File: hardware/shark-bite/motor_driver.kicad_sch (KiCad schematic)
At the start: 53 parts, among them J2 Conn_ARM_SWD_TagConnect_TC203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, J3 PWM Pads, J6 Motor Pads, U10 SISS54, U11 SISS54, U12 SISS54, U2 DRV8300DRGER, U4 GD32E230G6U6TR, U7 SISS54, U8 SISS54, U9 SISS54

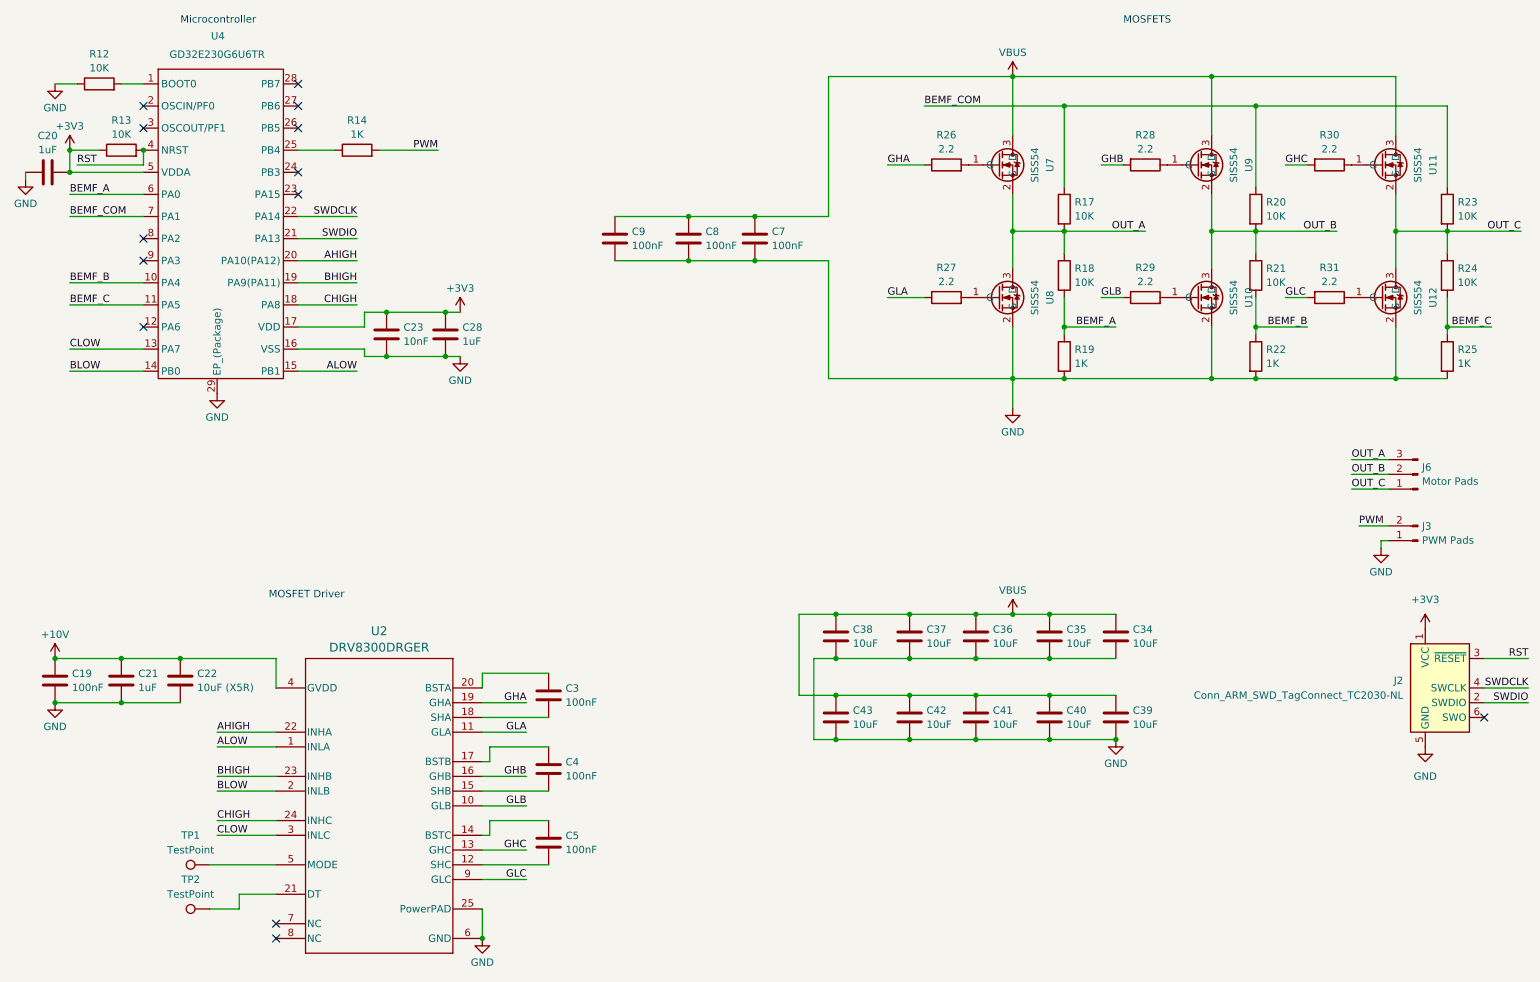
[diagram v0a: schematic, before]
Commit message: Minor Changes???
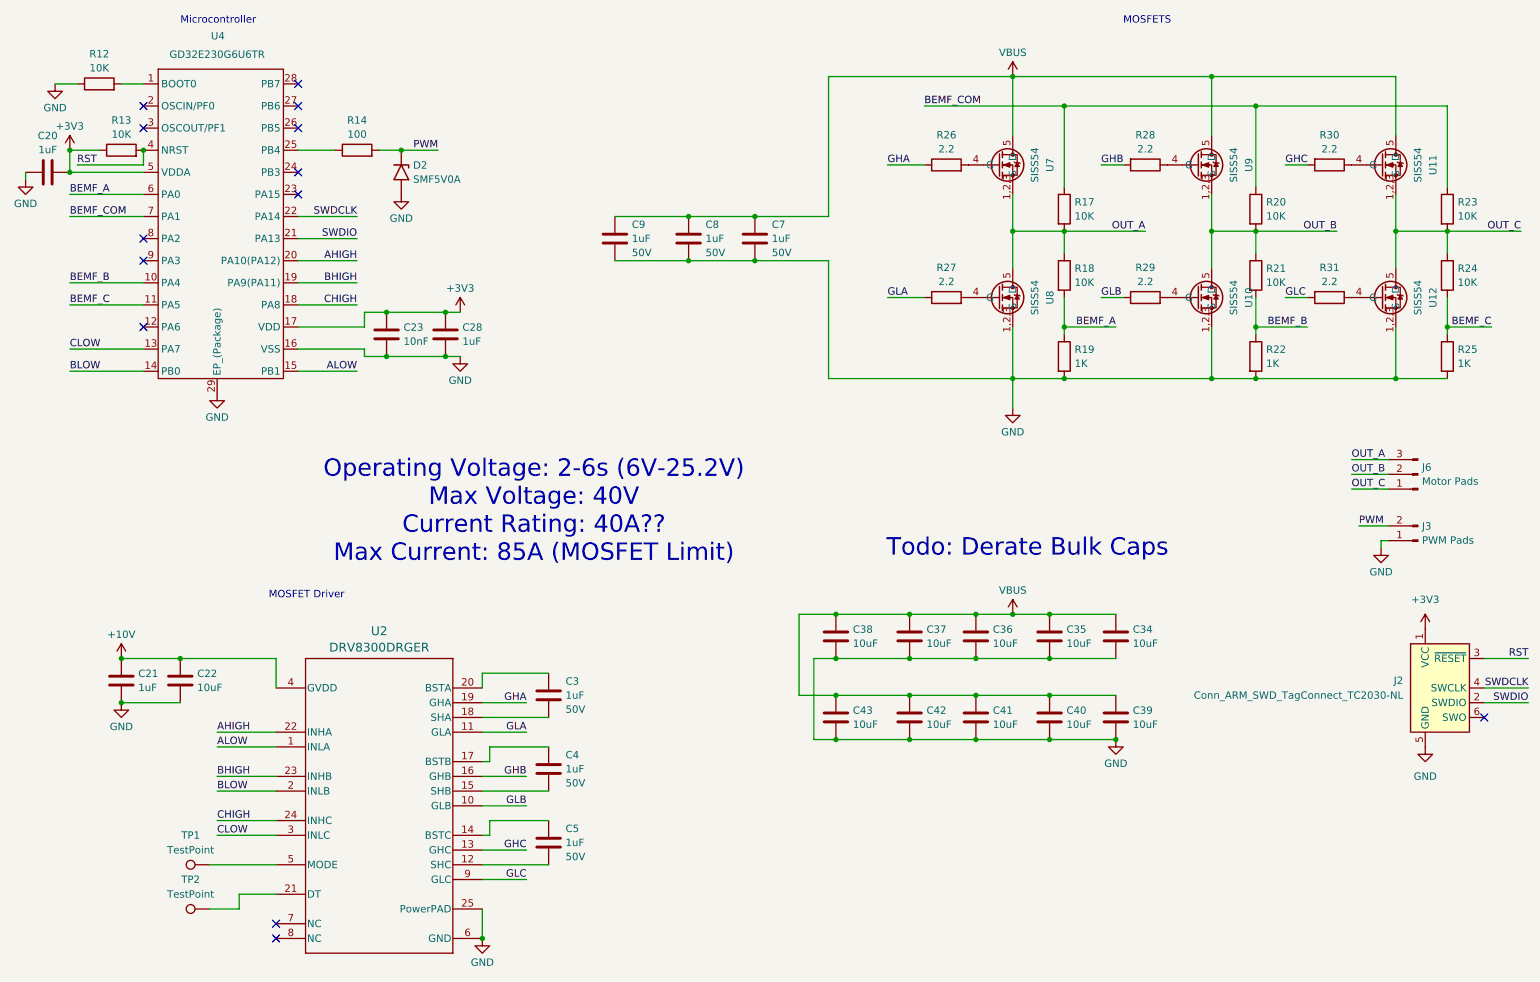
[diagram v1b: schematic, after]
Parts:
- removed C19: 100nF, Capacitor_SMD:C_0402_1005Metric_Pad0.74x0.62mm_HandSolder, symbol Device:C
- added D2: SMF5V0A, Diode_SMD:D_SMF, symbol Diode:SMF5V0A
- C20, C21: LCSC C7472948 -> (none)
- C22: value 10uF (X5R) -> 10uF; LCSC C2858031 -> (none)
- C23: LCSC C307331 -> (none)
- C28: LCSC C2858031 -> (none)
- C3, C4, C5: value 100nF -> 1uF; footprint Capacitor_SMD:C_0402_1005Metric_Pad0.74x0.62mm_HandSolder -> Capacitor_SMD:C_0603_1608Metric; LCSC C7472948 -> C307331; Vmax (none) -> 50V
- C7, C8, C9: value 100nF -> 1uF; footprint Capacitor_SMD:C_0603_1608Metric -> Capacitor_SMD:C_0402_1005Metric; LCSC (none) -> C307331; Vmax (none) -> 50V
- J3: footprint (none) -> Connector_PinHeader_1.00mm:PinHeader_1x02_P1.00mm_Vertical
- R14: value 1K -> 100; LCSC C11702 -> (none)
- TP1, TP2: footprint (none) -> TestPoint:TestPoint_Pad_1.0x1.0mm
- U10, U11, U12, U7, U8, U9: footprint Package_DFN_QFN:Infineon_PQFN-22-15-4EP_6x5mm_P0.65mm -> Sharkbite:1212-8S; Vmax (none) -> 40V
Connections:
- net GND: now also U10.1,2,3 (S), U12.1,2,3 (S), U8.1,2,3 (S), D2.2 (A2); no longer U10.2 (S), U12.2 (S), U8.2 (S)
- net OUT_A: now also U7.1,2,3 (S), U8.5 (D); no longer U7.2 (S), U8.3 (D)
- net OUT_B: now also U10.5 (D), U9.1,2,3 (S); no longer U10.3 (D), U9.2 (S)
- net OUT_C: now also U11.1,2,3 (S), U12.5 (D); no longer U11.2 (S), U12.3 (D)
- net PWM: now also D2.1 (A1)
- net VBUS: now also U11.5 (D), U7.5 (D), U9.5 (D); no longer U11.3 (D), U7.3 (D), U9.3 (D)
- net at R31.1: now also U12.4 (G); no longer U12.1 (G)
- net at R27.2: now also U8.4 (G); no longer U8.1 (G)
- net at R28.1: now also U9.4 (G); no longer U9.1 (G)
- net at R26.2: now also U7.4 (G); no longer U7.1 (G)
- net at R30.1: now also U11.4 (G); no longer U11.1 (G)
- net at R29.2: now also U10.4 (G); no longer U10.1 (G)
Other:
- note added: "Operating Voltage: 2-6s (6V-25.2V) Max Voltage: 40V Current Rating: 40A?? Max Current: 85A (MOSFET Limit)"
- note added: "Todo: Derate Bulk Caps"
- moved on the sheet: U10, U11, U12, U7, U8, U9

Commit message: Design Finished
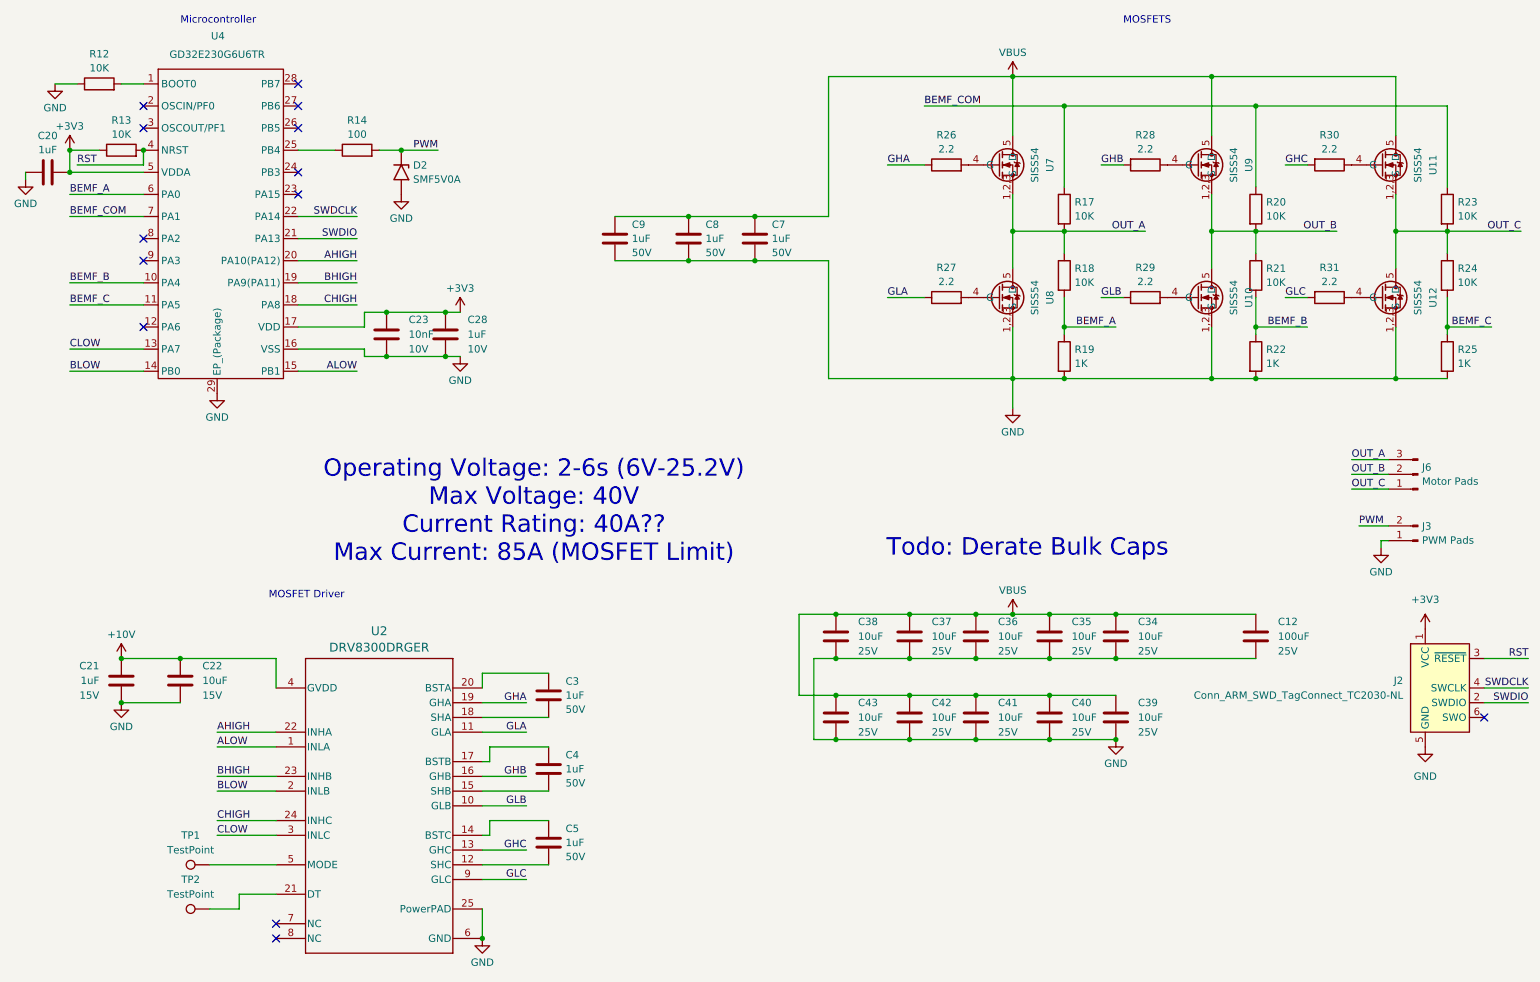
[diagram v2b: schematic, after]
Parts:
- added C12: 100uF, symbol Device:C
- C21, C22: Vmax (none) -> 15V
- C23, C28: Vmax (none) -> 10V
- C34, C35, C36, C37, C38, C39, C40, C41, C42, C43: Vmax (none) -> 25V
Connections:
- net GND: now also C12.2
- net VBUS: now also C12.1

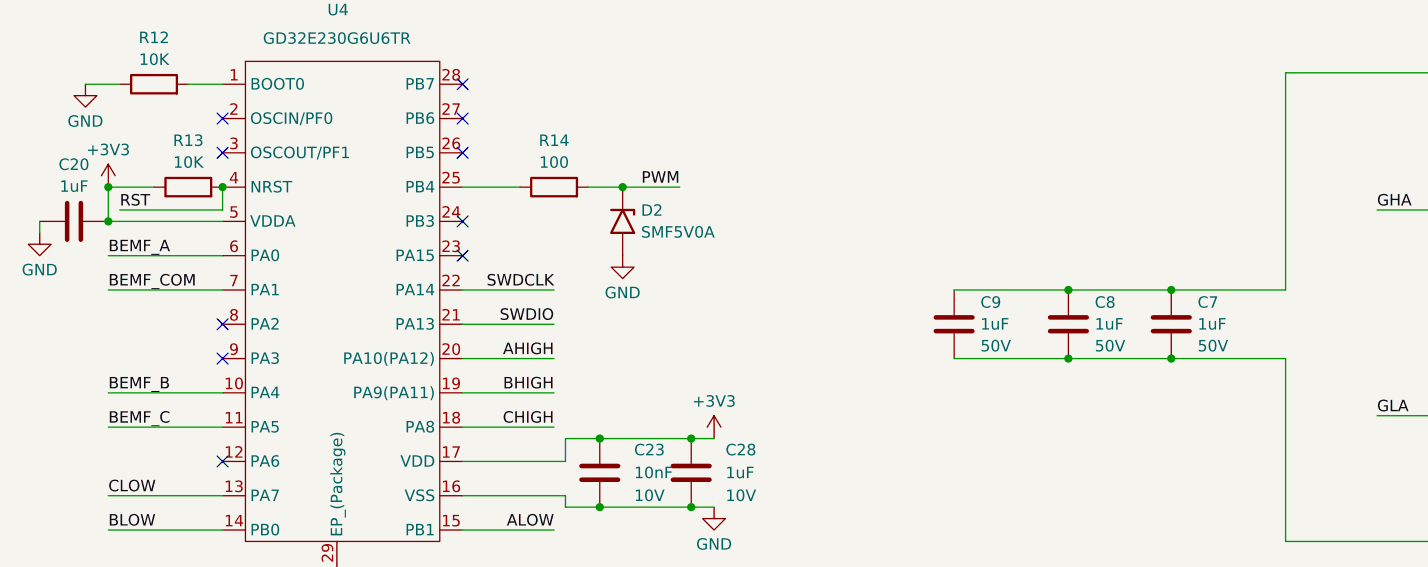
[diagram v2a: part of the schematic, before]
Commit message: Update JLC Files
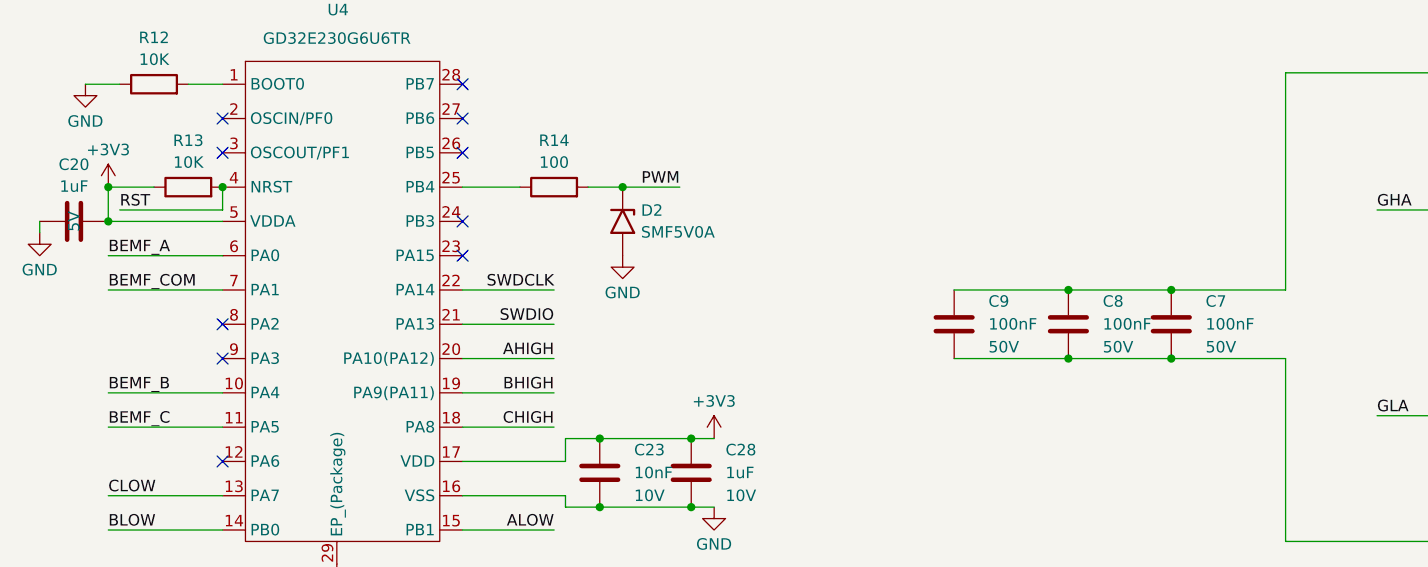
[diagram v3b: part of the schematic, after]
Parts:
- C20: Vmax (none) -> 5V
- C7, C8, C9: value 1uF -> 100nF
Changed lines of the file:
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@@
 			)
 		)
-		(property "Vmax" ""
+		(property "Vmax" "5V"
 			(at 26.67 46.99 0)
 			(effects
@@
 		(fields_autoplaced yes)
 		(property "Reference" "C8"
-			(at 140.081 55.9957 0)
-			(effects
-				(font
-					(size 1.27 1.27)
-				)
-				(justify left)
-			)
-		)
-		(property "Value" "1uF"
-			(at 140.081 58.42 0)
+			(at 140.97 55.8799 0)
+			(effects
+				(font
+					(size 1.27 1.27)
+				)
+				(justify left)
+			)
+		)
+		(property "Value" "100nF"
+			(at 140.97 58.4199 0)
 			(effects
 				(font
@@
 		)
 		(property "Vmax" "50V"
-			(at 140.081 60.8443 0)
+			(at 140.97 60.9599 0)
 			(effects
 				(font
@@
 		(fields_autoplaced yes)
 		(property "Reference" "C9"
-			(at 127.381 55.9957 0)
-			(effects
-				(font
-					(size 1.27 1.27)
-				)
-				(justify left)
-			)
-		)
-		(property "Value" "1uF"
-			(at 127.381 58.42 0)
+			(at 128.27 55.8799 0)
+			(effects
+				(font
+					(size 1.27 1.27)
+				)
+				(justify left)
+			)
+		)
+		(property "Value" "100nF"
+			(at 128.27 58.4199 0)
 			(effects
 				(font
@@
 		)
 		(property "Vmax" "50V"
-			(at 127.381 60.8443 0)
+			(at 128.27 60.9599 0)
 			(effects
 				(font
@@
 		(fields_autoplaced yes)
 		(property "Reference" "C7"
-			(at 151.511 55.9957 0)
-			(effects
-				(font
-					(size 1.27 1.27)
-				)
-				(justify left)
-			)
-		)
-		(property "Value" "1uF"
-			(at 151.511 58.42 0)
+			(at 152.4 55.8799 0)
+			(effects
+				(font
+					(size 1.27 1.27)
+				)
+				(justify left)
+			)
+		)
+		(property "Value" "100nF"
+			(at 152.4 58.4199 0)
 			(effects
 				(font
@@
 		)
 		(property "Vmax" "50V"
-			(at 151.511 60.8443 0)
-			(effects
-				(font
+			(at 152.4 60.9599 0)
+			(effects
+				(font
